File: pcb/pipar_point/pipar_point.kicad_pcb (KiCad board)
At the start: 2 copper layers, 145.3 x 110.3 mm, 116 parts, among them Q1 AO3416 N-channel MOSFET, SW1 SW_Wuerth_450301014042, SW2 CK_KMS2xxG, U1 Seeeduino Xiao nRF52840, U2 74HC595

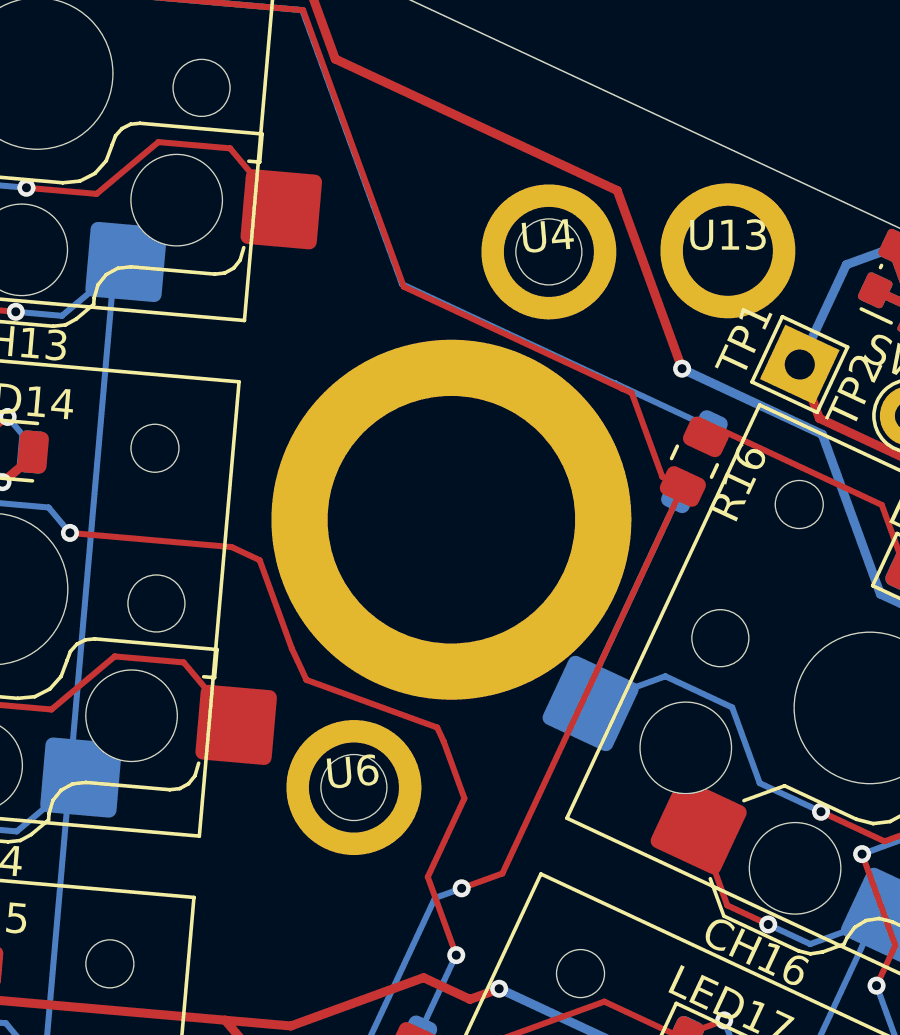
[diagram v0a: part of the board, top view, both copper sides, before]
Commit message: moves the through hole away from pad
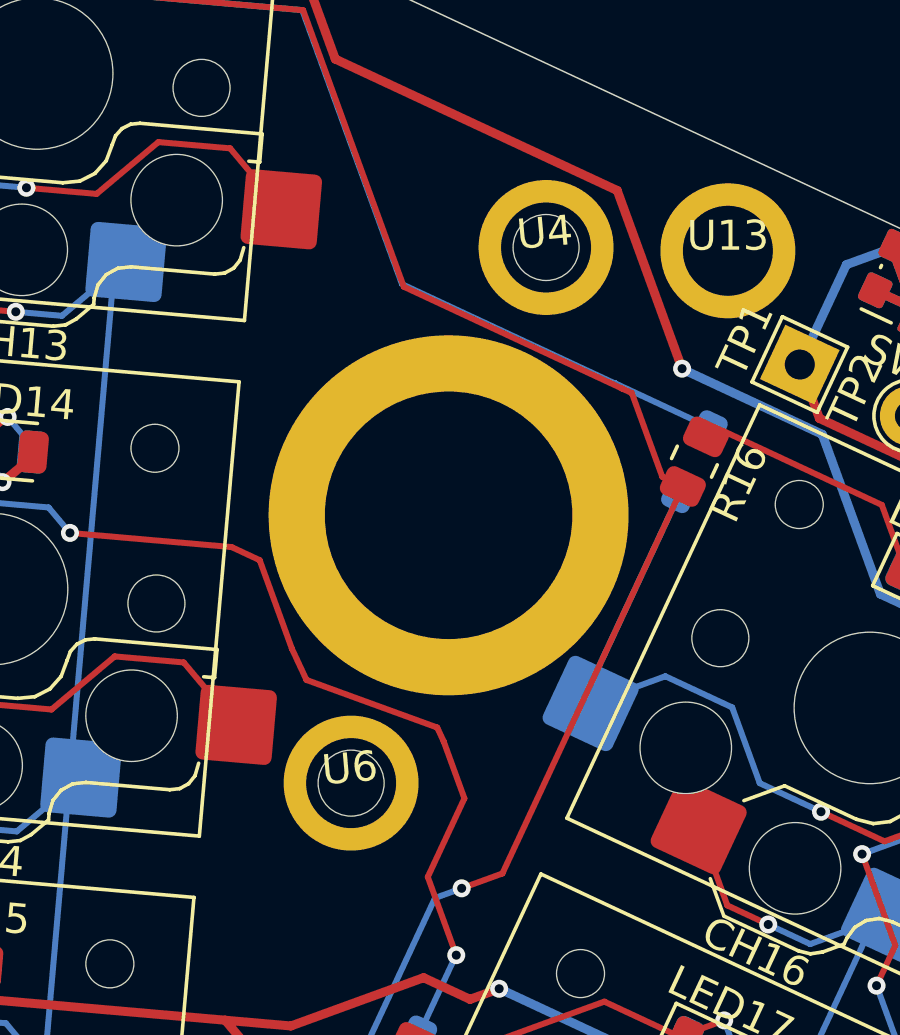
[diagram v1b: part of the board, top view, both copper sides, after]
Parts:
- moved U4 0.17 mm to (200.7, 50.2)
- moved U5 0.17 mm to (197.4, 59.1)
- moved U6 0.17 mm to (194.2, 68.1)
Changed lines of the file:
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@@
 	(footprint "choc:Solder Nut"
 		(layer "F.Cu")
-		(at 200.763496 50.356872 5)
+		(at 200.669999 50.210003 5)
 		(property "Reference" "U4"
 			(at 0 -0.5 5)
@@
 	(footprint "choc:Trackpoint_T460s_Stick"
 		(layer "F.Cu")
-		(at 197.514306 59.283949 -20)
+		(at 197.420809 59.13708 -20)
 		(property "Reference" "U5"
 			(at 0 12.7 -20)
@@
 	(footprint "choc:Solder Nut"
 		(layer "F.Cu")
-		(at 194.265111 68.211063 5)
+		(at 194.171614 68.064194 5)
 		(property "Reference" "U6"
 			(at 0 -0.5 5)
